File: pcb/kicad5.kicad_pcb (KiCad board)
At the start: 2 copper layers, 42.9 x 59.8 mm, 8 parts, among them SW1 SW_Push, SW2 SW_Push, SW3 SW_Push, SW4 SW_Push, SW5 RotaryEncoder_Switch, U1 XIAO-RP2040-DIP

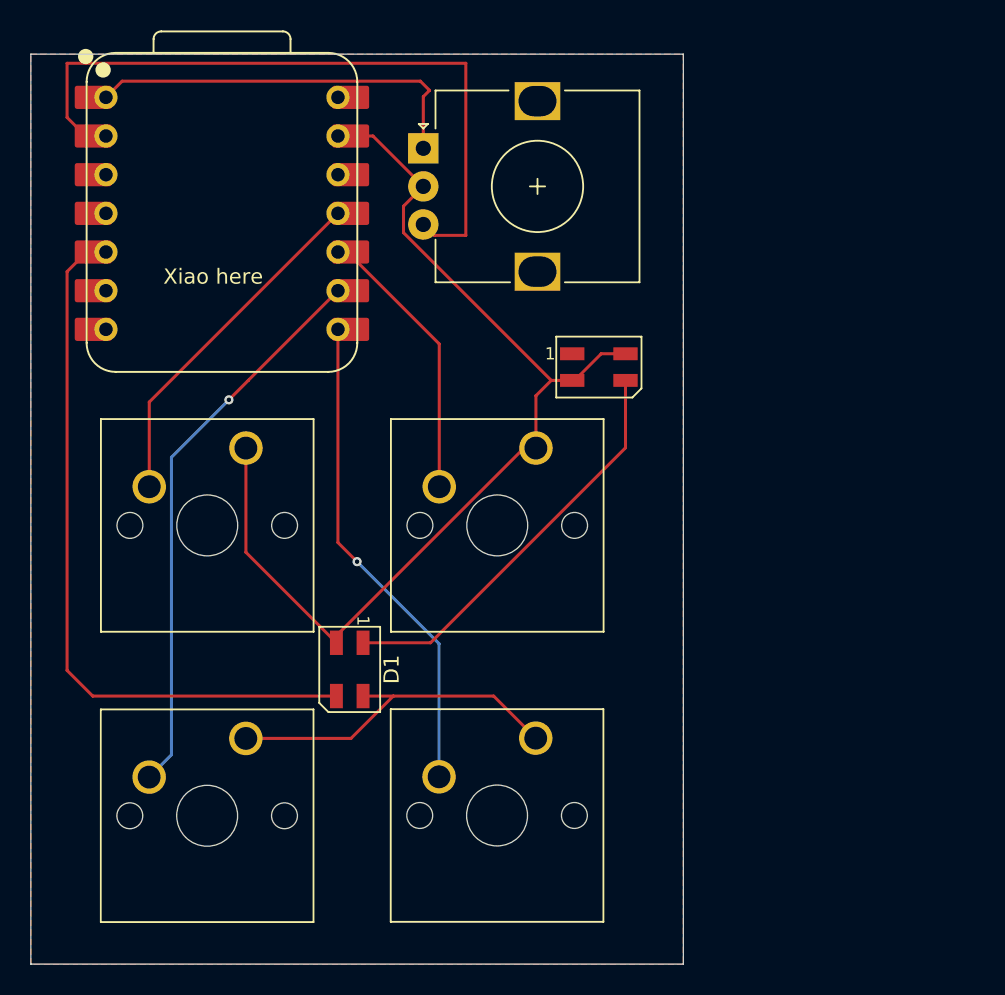
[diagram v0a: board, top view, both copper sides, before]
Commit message: chnges
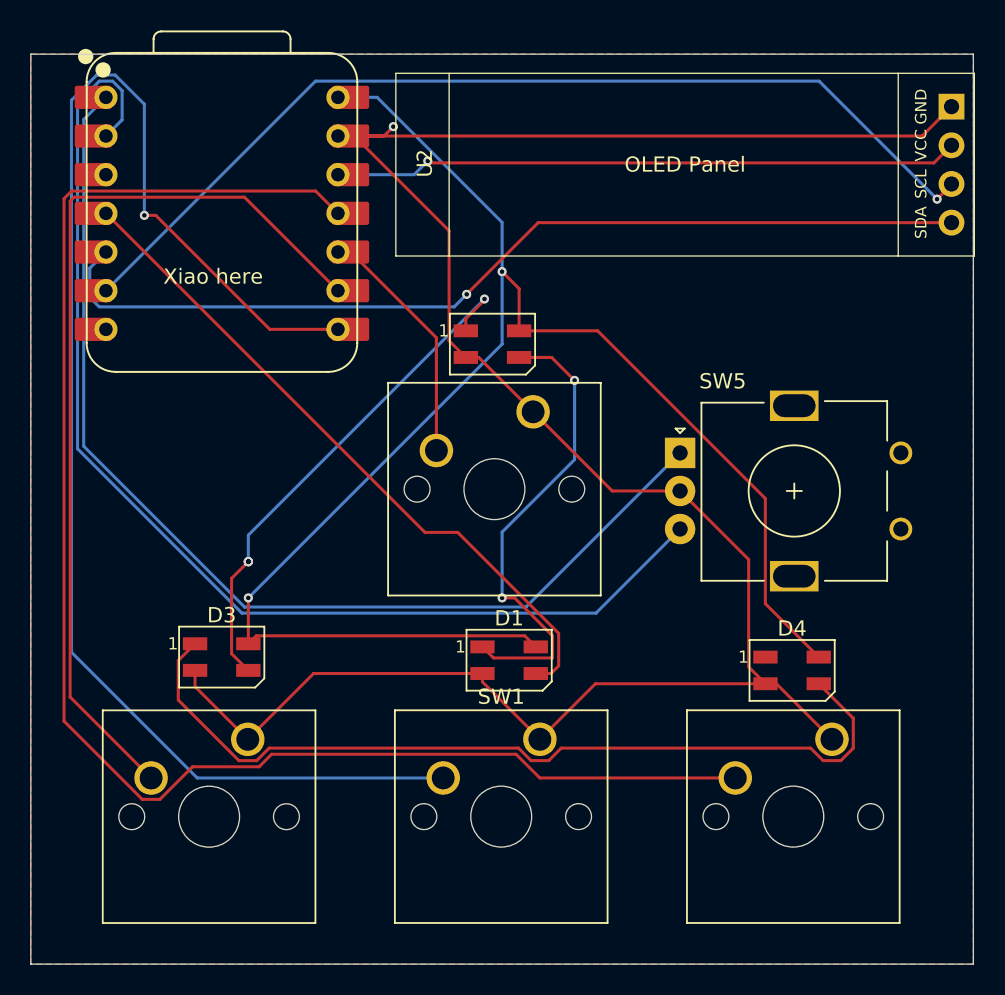
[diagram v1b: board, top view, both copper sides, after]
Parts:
- added D3: SK6812MINI, LED_SMD:LED_SK6812MINI_PLCC4_3.5x3.5mm_P1.75mm, F.Cu at (150.7, 111.0)
- added D4: SK6812MINI, LED_SMD:LED_SK6812MINI_PLCC4_3.5x3.5mm_P1.75mm, F.Cu at (188.1, 111.9)
- added U2: SSD1306, Oled:SSD1306-0.91-OLED-4pin-128x32, F.Cu at (162.1, 72.7)
- SW5: footprint ec11:RotaryEncoder_Alps_EC12E_Vertical_H20mm -> ec11:RotaryEncoder_Alps_EC11E_Vertical_H20mm
- moved SW4 43.0 mm to (190.7, 116.4)
- moved SW5 26.2 mm to (180.8, 97.6)
- moved D1 10.5 mm to (169.5, 111.2), turned to 0 degrees
- moved D2 7.15 mm to (168.4, 90.5)
- moved SW3 2.39 mm to (171.1, 94.9)
- moved SW1 0.28 mm to (171.6, 116.4)
- moved SW2 0.14 mm to (152.4, 116.4)
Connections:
- D1 pad 4: GND -> +5V
- D2 pad 1: unconnected-(D2-DOUT-Pad1) -> Net-(D2-DOUT)
- D2 pad 4: GND -> +5V
- U1 pad 12: unconnected-(U1-3V3-Pad12) -> +3.3V
- U1 pad 4: unconnected-(U1-GPIO29/ADC3/A3-Pad4) -> Net-(D1-DIN)
- U1 pad 5: Net-(D1-DIN) -> Net-(U1-GPIO6/SDA)
- U1 pad 6: unconnected-(U1-GPIO7/SCL-Pad6) -> Net-(U1-GPIO7/SCL)
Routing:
- net +5V: track 0.00 -> 105.1 mm, vias 0 -> 2
- net Net-(U1-GPIO3/MOSI): track 23.1 -> 101.2 mm
- net Net-(U1-GPIO7/SCL): track 0.00 -> 64.8 mm, vias 0 -> 1
- net Net-(U1-GPIO6/SDA): track 0.00 -> 62.6 mm, vias 0 -> 1
- net Net-(U1-GPIO1/RX): track 32.1 -> 93.4 mm
- net Net-(D3-DOUT): track 0.00 -> 57.0 mm
- net GND: track 92.0 -> 147.6 mm, vias 0 -> 1
- net Net-(U1-GPIO26/ADC0/A0): track 25.9 -> 71.3 mm
- net +3.3V: track 0.00 -> 41.0 mm, vias 0 -> 1
- net Net-(D2-DOUT): track 0.00 -> 34.4 mm, vias 0 -> 4
- net Net-(U1-GPIO27/ADC1/A1): track 47.2 -> 76.3 mm
- net Net-(U1-GPIO2/SCK): track 37.9 -> 60.3 mm, vias 1 -> 0
- net Net-(D1-DOUT): track 27.0 -> 31.2 mm, vias 0 -> 2
- net Net-(D1-DIN): track 47.7 -> 45.0 mm
- net Net-(U1-GPIO4/MISO): track 18.5 -> 16.2 mm
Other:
- board size 42.9 x 59.8 mm -> 61.9 x 59.8 mm
